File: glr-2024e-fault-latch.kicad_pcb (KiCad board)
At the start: 2 copper layers, 110 x 90 mm, 70 parts, among them K101 Fujitsu_FTR-LYAA005x, K103 Fujitsu_FTR-LYAA005x, Q101 Q_NPN_BEC, Q102 Q_NPN_BEC, Q103 Q_NPN_BEC, Q104 Q_NPN_BEC, Q105 Q_NMOS_GSD, Q106 Q_NMOS_GSD, Q107 Q_PMOS_GSD, Q108 Q_PMOS_GSD, Q114 Q_NMOS_GSD, Q115 Q_NMOS_GSD, SW101 SW_Omron_B3FS, SW102 SW_Omron_B3FS, U101 SFH617A-1, U102 SFH617A-1, U104 74AHC1G00, U105 74AHC1G00, U107 74LS279, U108 641964-1, U109 SFH617A-1, U110 SFH617A-1, U112 641964-1, U115 641964-1, U116 641964-1, U120 641964-1, U123 641964-1

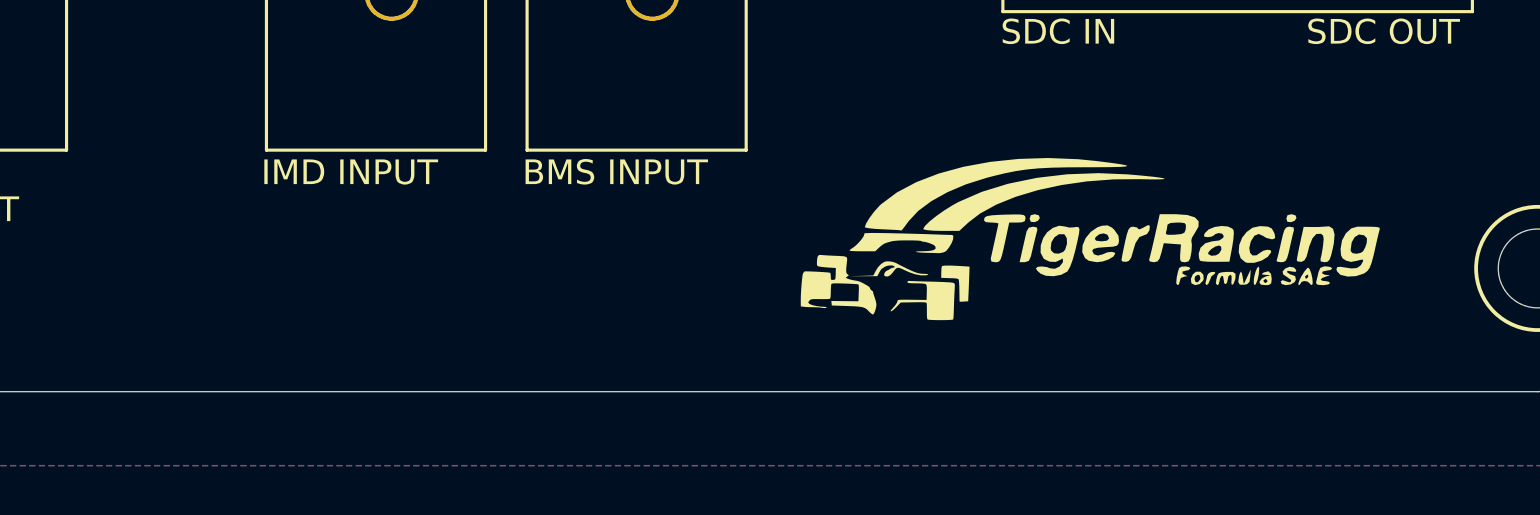
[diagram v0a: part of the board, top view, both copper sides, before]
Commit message: add glr logo
Co-Authored-By: wallalex0 <97884125+wallalex0@users.noreply.github.com>
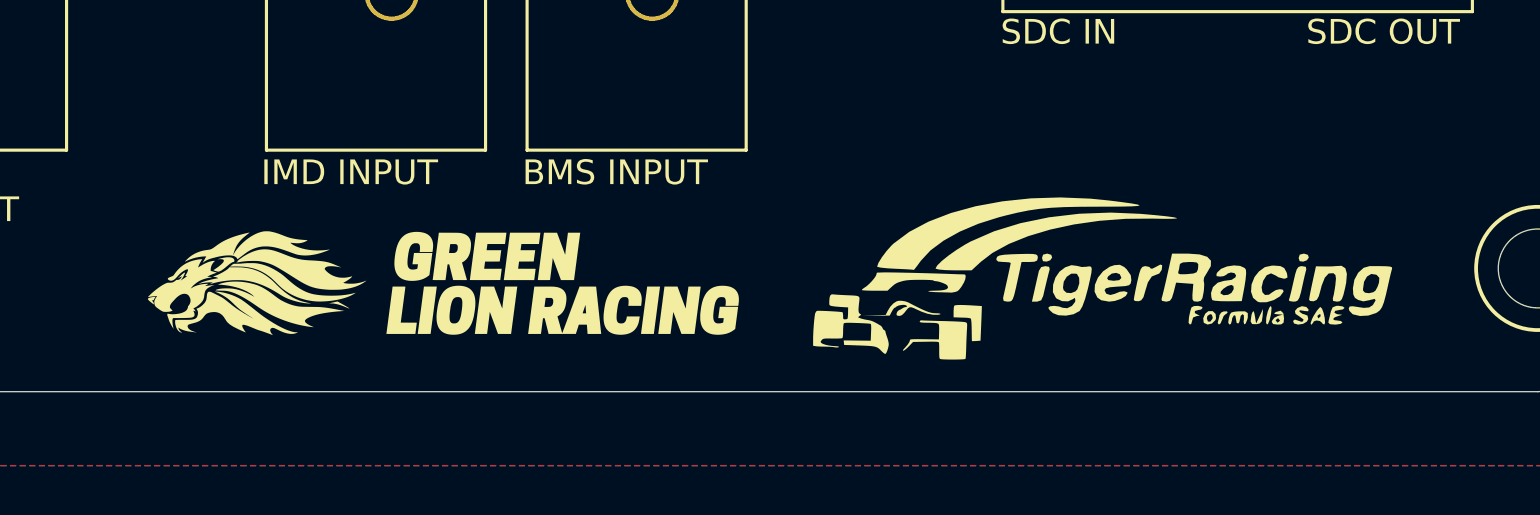
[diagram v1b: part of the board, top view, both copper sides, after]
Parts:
- added G***: LOGO, GLR_KiCAD_Library:glr-logo, F.Cu at (129.8, 129.7)
- moved G*** 1.68 mm to (156.5, 129.6)
- moved G*** 1.68 mm to (148.3, 131.0)
